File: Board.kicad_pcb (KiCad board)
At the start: 2 copper layers, 101.6 x 53.3 mm, 17 parts, among them P1 Relay 1, P10 CONN_01X18, P11 CONN_01X18, P12 CONN_01X06, P2 Relay 2, P3 Relay 3, P4 Relay 4, P5 CONN_01X08, P6 CONN_01X08, P7 CONN_01X08, P8 CONN_01X08, P9 CONN_01X08

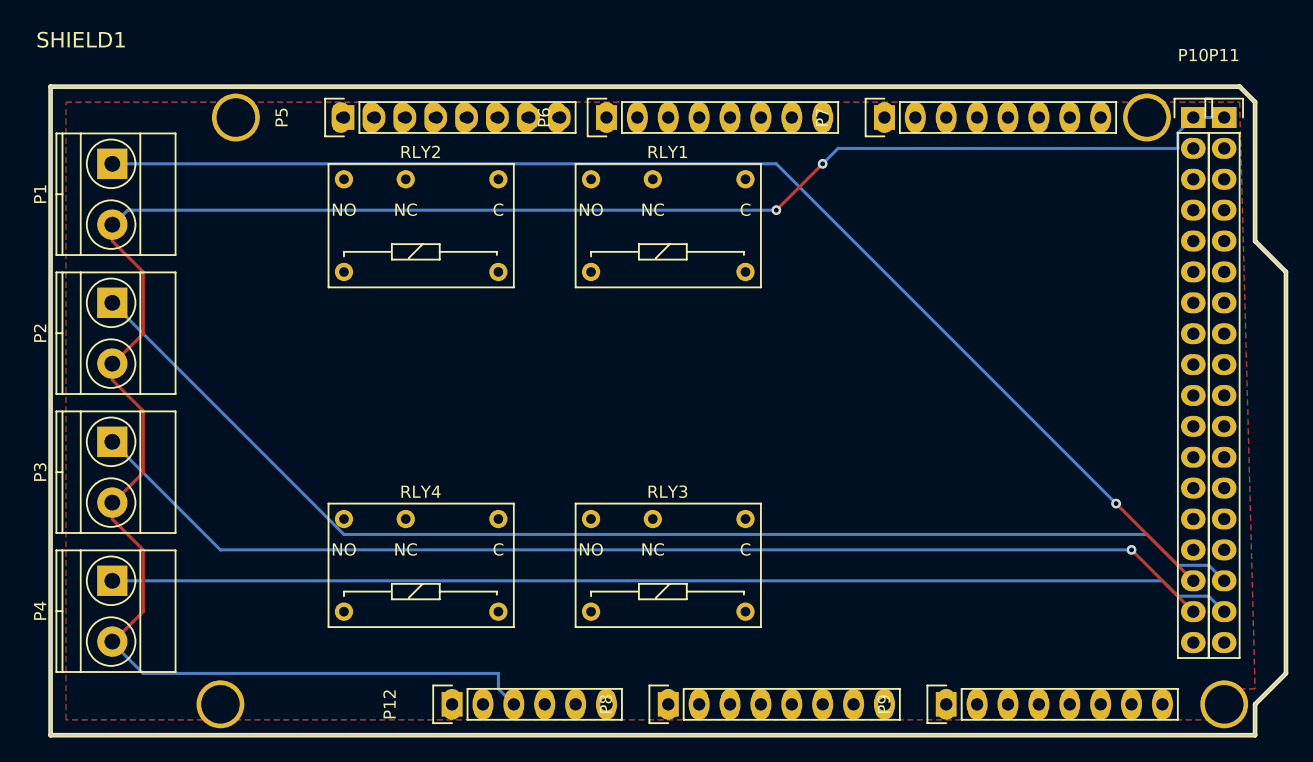
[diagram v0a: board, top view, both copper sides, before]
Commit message: Cleaning Up Board
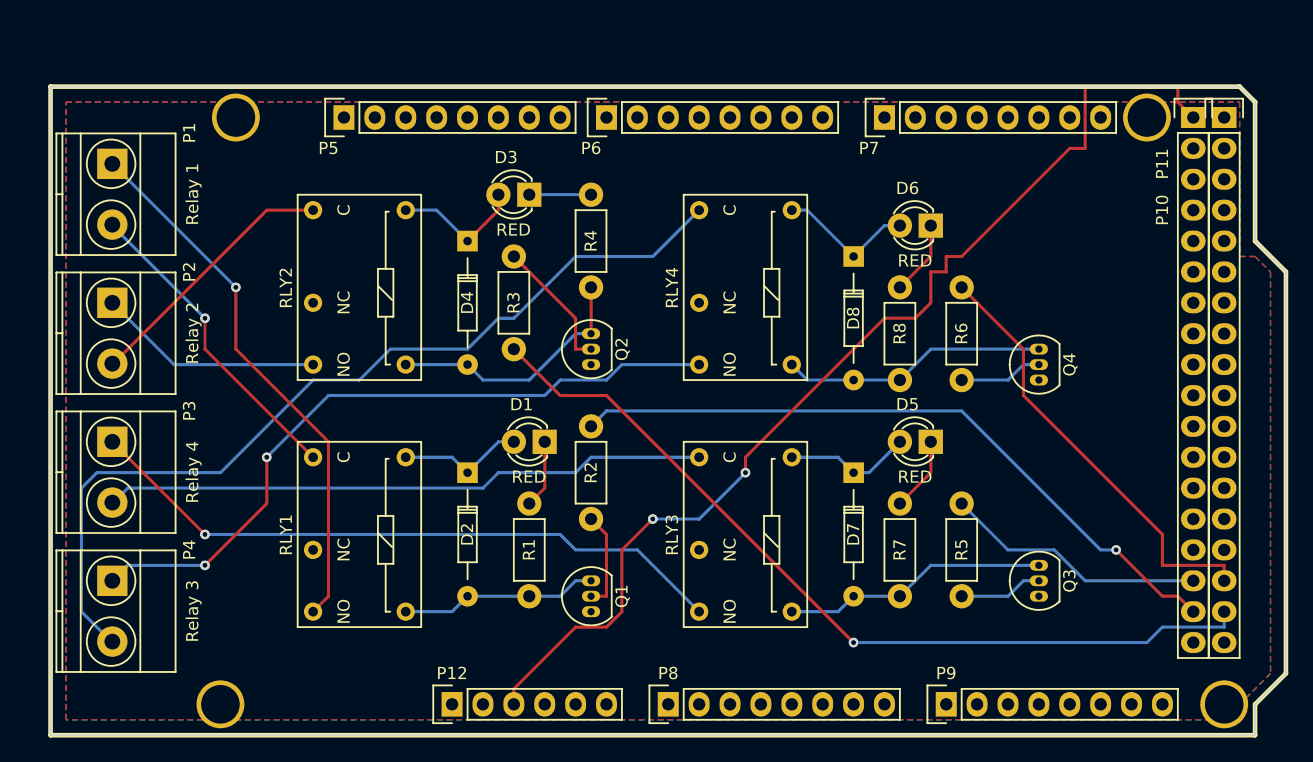
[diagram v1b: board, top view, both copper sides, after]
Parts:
- added D1: RED, LEDs:LED-3MM, F.Cu at (154.9, 115.6)
- added D2: 1N4148, Diodes_ThroughHole:Diode_DO-35_SOD27_Horizontal_RM10, F.Cu at (148.6, 118.1)
- added D3: RED, LEDs:LED-3MM, F.Cu at (153.7, 95.2)
- added D4: 1N4148, Diodes_ThroughHole:Diode_DO-35_SOD27_Horizontal_RM10, F.Cu at (148.6, 99.1)
- added D5: RED, LEDs:LED-3MM, F.Cu at (186.7, 115.6)
- added D6: RED, LEDs:LED-3MM, F.Cu at (186.7, 97.8)
- added D7: 1N4148, Diodes_ThroughHole:Diode_DO-35_SOD27_Horizontal_RM10, F.Cu at (180.3, 118.1)
- added D8: 1N4148, Diodes_ThroughHole:Diode_DO-35_SOD27_Horizontal_RM10, F.Cu at (180.3, 100.3)
- added Q1: PN2222A, TO_SOT_Packages_THT:TO-92_Inline_Narrow_Oval, F.Cu at (158.8, 129.5)
- added Q2: PN2222A, TO_SOT_Packages_THT:TO-92_Inline_Narrow_Oval, F.Cu at (158.8, 109.2)
- added Q3: PN2222A, TO_SOT_Packages_THT:TO-92_Inline_Narrow_Oval, F.Cu at (195.6, 128.3)
- added Q4: PN2222A, TO_SOT_Packages_THT:TO-92_Inline_Narrow_Oval, F.Cu at (195.6, 110.5)
- added R1: 470, Resistors_ThroughHole:Resistor_Horizontal_RM7mm, F.Cu at (153.7, 120.7)
- added R2: 2.2K, Resistors_ThroughHole:Resistor_Horizontal_RM7mm, F.Cu at (158.8, 121.9)
- added R3: 2.2K, Resistors_ThroughHole:Resistor_Horizontal_RM7mm, F.Cu at (152.4, 100.3)
- added R4: 470, Resistors_ThroughHole:Resistor_Horizontal_RM7mm, F.Cu at (158.8, 95.2)
- added R5: 2.2K, Resistors_ThroughHole:Resistor_Horizontal_RM7mm, F.Cu at (189.2, 128.3)
- added R6: 2.2K, Resistors_ThroughHole:Resistor_Horizontal_RM7mm, F.Cu at (189.2, 110.5)
- added R7: 470, Resistors_ThroughHole:Resistor_Horizontal_RM7mm, F.Cu at (184.2, 120.7)
- added R8: 470, Resistors_ThroughHole:Resistor_Horizontal_RM7mm, F.Cu at (184.2, 102.9)
- P3: value Relay 3 -> Relay 4
- P4: value Relay 4 -> Relay 3
- RLY1, RLY2, RLY3, RLY4: value G6E-134P-US DC5 -> RELAY_40.31; footprint Relays_THT:Relay_SPDS_OMRON-G6E -> Relays_ThroughHole:Relay_SPDS_OMRON-G6E
- moved RLY4 42.1 mm to (175.3, 109.2), turned to 90 degrees
- moved RLY1 31.8 mm to (143.5, 129.5), turned to 90 degrees
- moved RLY3 16.5 mm to (175.3, 129.5), turned to 90 degrees
- moved RLY2 9.16 mm to (143.5, 109.2), turned to 90 degrees
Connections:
- P1 pad 1: Relay1 -> Net-(P1-Pad1)
- P1 pad 2: 5V -> Net-(P1-Pad2)
- P10 pad 16: Relay1 -> Relay3
- P10 pad 17: Relay3 -> Relay1
- P11 pad 16: Relay2 -> Relay4
- P11 pad 17: Relay4 -> Relay2
- P2 pad 1: Relay2 -> Net-(P2-Pad1)
- P2 pad 2: 5V -> Net-(P2-Pad2)
- P3 pad 1: Relay3 -> Net-(P3-Pad1)
- P3 pad 2: 5V -> Net-(P3-Pad2)
- P4 pad 1: Relay4 -> Net-(P4-Pad1)
- P4 pad 2: 5V -> Net-(P4-Pad2)
- RLY1 pad 10: (no net) -> Net-(RLY1-Pad10)
- RLY1 pad 12: Net-(RLY1-Pad12) -> Net-(P1-Pad1)
- RLY1 pad 6: (no net) -> Net-(D1-Pad2)
- RLY1 pad 7: (no net) -> Net-(P1-Pad2)
- RLY2 pad 10: (no net) -> Net-(RLY2-Pad10)
- RLY2 pad 12: Net-(RLY2-Pad12) -> Net-(P2-Pad1)
- RLY2 pad 6: (no net) -> Net-(D3-Pad2)
- RLY2 pad 7: (no net) -> Net-(P2-Pad2)
- RLY3 pad 10: (no net) -> Net-(RLY3-Pad10)
- RLY3 pad 12: Net-(RLY3-Pad12) -> Net-(P3-Pad1)
- RLY3 pad 6: (no net) -> Net-(D5-Pad2)
- RLY3 pad 7: (no net) -> Net-(P3-Pad2)
- RLY4 pad 10: (no net) -> Net-(RLY4-Pad10)
- RLY4 pad 12: Net-(RLY4-Pad12) -> Net-(P4-Pad1)
- RLY4 pad 6: (no net) -> Net-(D6-Pad2)
- RLY4 pad 7: (no net) -> Net-(P4-Pad2)
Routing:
- net 5V: track 173.0 -> 88.4 mm
- net Net-(P4-Pad2): track 0.00 -> 74.1 mm
- net Relay3: track 94.7 -> 21.7 mm, vias 1 -> 0
- net Net-(P4-Pad1): track 0.00 -> 57.9 mm, vias 0 -> 2
- net Relay4: track 92.5 -> 36.0 mm
- net Net-(P3-Pad1): track 0.00 -> 54.0 mm, vias 0 -> 1
- net Net-(P3-Pad2): track 0.00 -> 49.9 mm
- net Relay1: track 103.1 -> 56.9 mm
- net Net-(P1-Pad1): track 0.00 -> 44.7 mm, vias 0 -> 1
- net Relay2: track 100.9 -> 70.2 mm, vias 0 -> 1
- net Net-(P1-Pad2): track 0.00 -> 26.0 mm, vias 0 -> 1
- net Net-(D8-Pad2): track 0.00 -> 21.9 mm
- net Net-(D7-Pad2): track 0.00 -> 21.9 mm
- net Net-(P2-Pad2): track 0.00 -> 21.9 mm
- net Net-(D4-Pad2): track 0.00 -> 21.2 mm
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- added copper zone on F.Cu, net 5V
- added copper zone on B.Cu, net GND
- removed copper zone on F.Cu, net GND

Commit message: Finishing up board
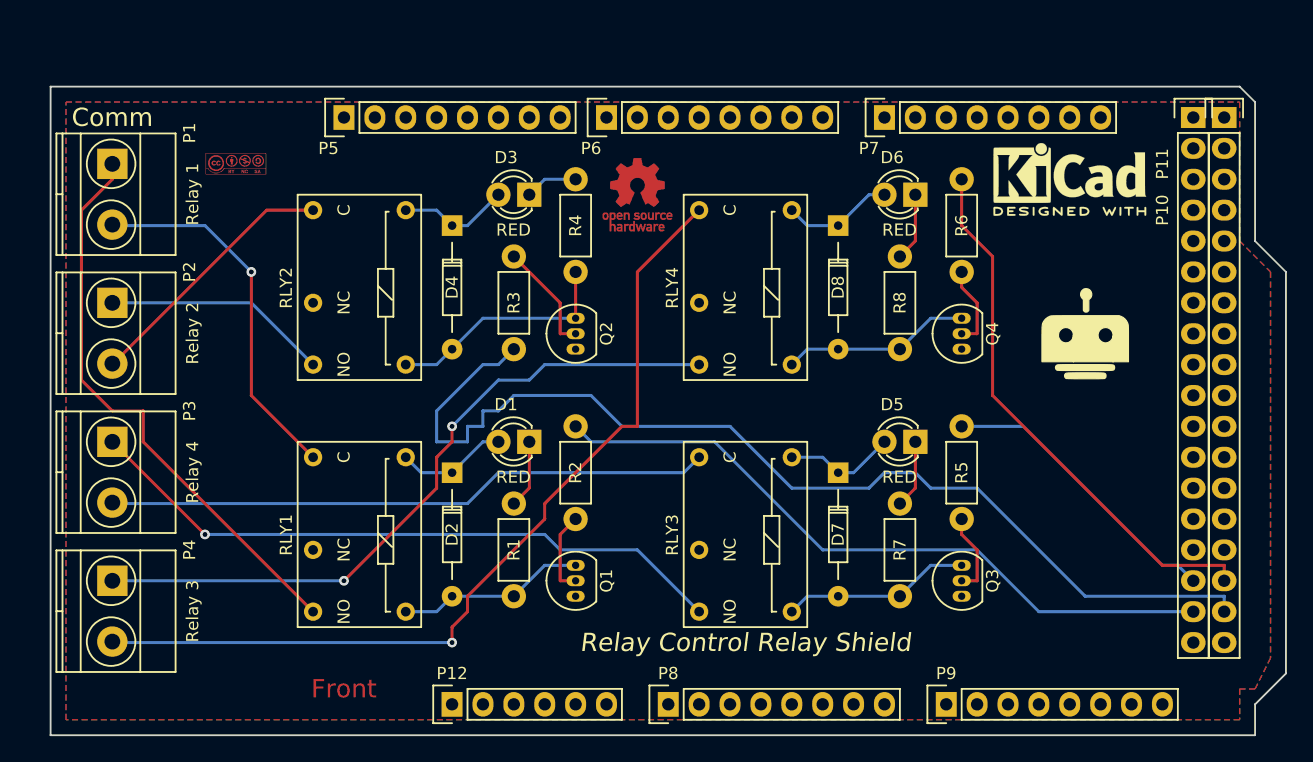
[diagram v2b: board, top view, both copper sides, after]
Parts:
- removed SHIELD1: ARDUINO_MEGA_SHIELD, arduino_shields:ARDUINO MEGA SHIELD
- added G***: LOGO, w_logo:Logo_copper_CC-BY-NC-SA_5x2mm, F.Cu at (129.5, 92.7)
- added G***: LOGO, freetronics_footprints:LOGO_NODEBOTS, F.Cu at (199.4, 106.7)
- added REF***: OSHW-Logo_5.7x6mm_Copper, Symbols:OSHW-Logo_5.7x6mm_Copper, F.Cu at (162.6, 95.2)
- added REF***: OSHW-Symbol_6.7x6mm_SilkScreen, Symbols:OSHW-Symbol_6.7x6mm_SilkScreen, B.Cu at (162.6, 95.2)
- added REF***: KiCad-Logo2_6mm_SilkScreen, Symbols:KiCad-Logo2_6mm_SilkScreen, F.Cu at (198.1, 94.0)
- moved R6 8.89 mm to (189.2, 101.6)
- moved Q4 6.84 mm to (189.2, 108.0)
- moved Q3 6.35 mm to (189.2, 128.3)
- moved R5 6.35 mm to (189.2, 121.9)
- moved D6 2.84 mm to (185.4, 95.2)
- moved D8 2.84 mm to (179.1, 97.8)
- moved R8 2.54 mm to (184.2, 100.3)
- moved D4 1.80 mm to (147.3, 97.8)
- moved Q2 1.80 mm to (157.5, 108.0)
- moved R4 1.80 mm to (157.5, 94.0)
- moved Q1 1.80 mm to (157.5, 128.3)
- moved D1 1.27 mm to (153.7, 115.6)
- moved D2 1.27 mm to (147.3, 118.1)
- moved D5 1.27 mm to (185.4, 115.6)
- moved D7 1.27 mm to (179.1, 118.1)
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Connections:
- P10 pad 1: 5V -> Net-(P10-Pad1)
- P11 pad 1: 5V -> Net-(P11-Pad1)
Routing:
- net 5V: track 88.4 -> 0.00 mm, vias 2 -> 0
- net Relay2: track 70.2 -> 88.0 mm, vias 1 -> 0
- net Relay4: track 36.0 -> 44.9 mm
- net Net-(D7-Pad2): track 21.9 -> 15.6 mm
- net Net-(D8-Pad2): track 21.9 -> 15.6 mm
- net Net-(P1-Pad2): track 26.0 -> 30.4 mm
- net Relay3: track 21.7 -> 24.3 mm
- net Net-(P1-Pad1): track 44.7 -> 47.3 mm, vias 1 -> 0
- net Net-(D6-Pad2): track 11.5 -> 9.20 mm
- net Net-(Q2-Pad2): track 11.0 -> 9.20 mm
- net Net-(D4-Pad2): track 21.2 -> 19.4 mm
- net Net-(D3-Pad2): track 11.0 -> 9.20 mm
- net Net-(P4-Pad2): track 74.1 -> 72.7 mm, vias 0 -> 1
- net Net-(Q1-Pad2): track 8.15 -> 6.88 mm
- net Net-(D1-Pad2): track 10.5 -> 9.20 mm
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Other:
- board text added: "Back"
- board text added: "Comm"
- board text added: "Front"
- board text added: "Relay Control Relay Shield"
